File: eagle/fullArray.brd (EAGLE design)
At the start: 40 x 70 mm, 120 parts

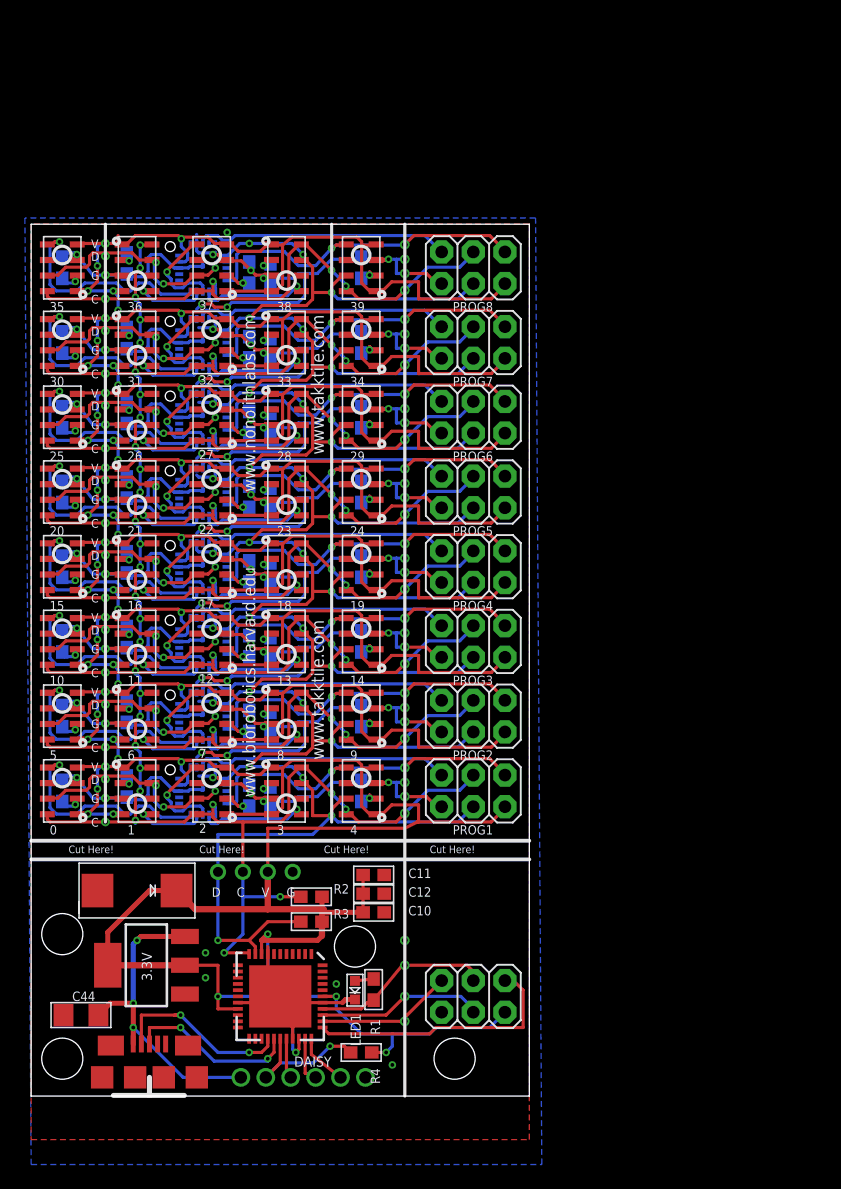
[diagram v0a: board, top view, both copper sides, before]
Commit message: need to tweak address pins, but should be manufacturable
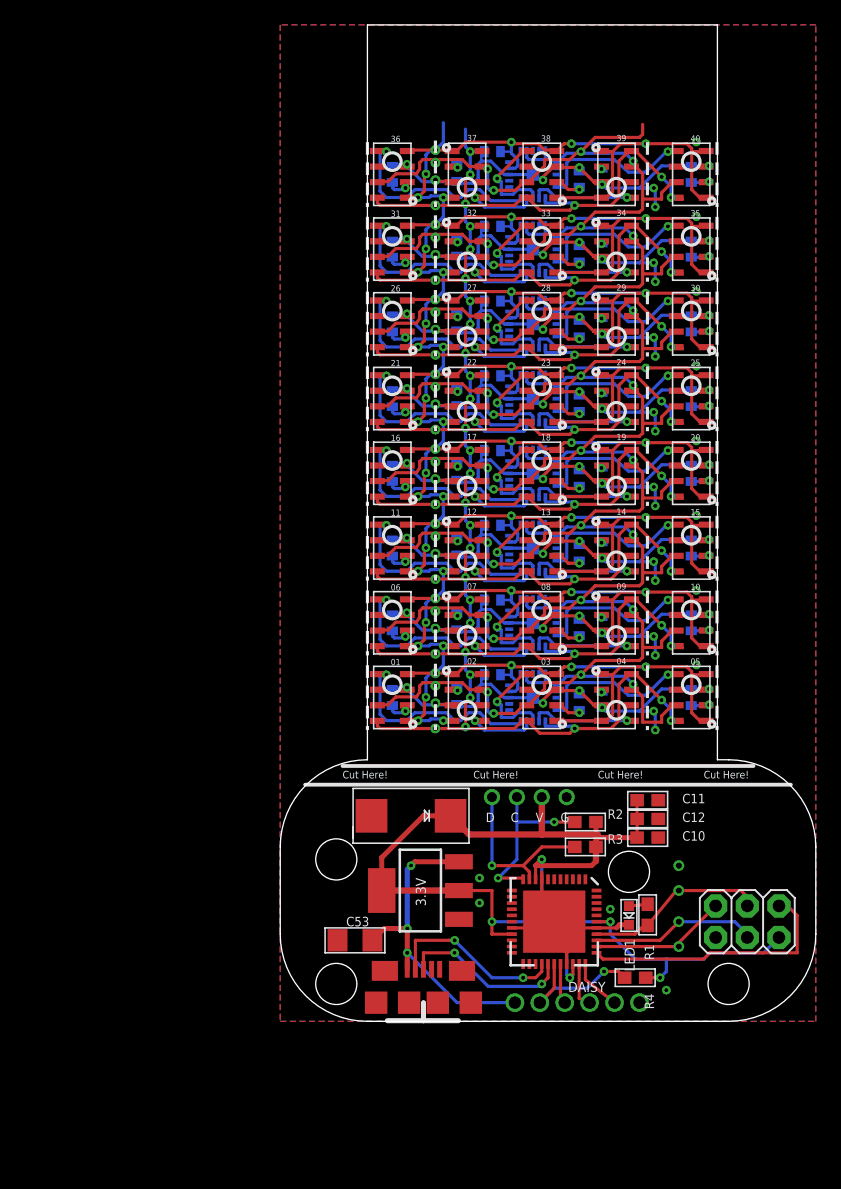
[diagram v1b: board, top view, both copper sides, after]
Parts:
- removed 0, 1, 2, 3, 4, 5, 6, 7, 8, 9: MPL115A2, nonolith:LGA-8
- removed AT1, AT2, AT3, AT4, AT5, AT6, AT7, AT8: ATTINYX4AMH, nonolith:QFN-20
- removed C0, C1, C2, C3, C4, C5, C7, C8, C9: 1uF, nonolith:0603
- removed PROG1, PROG2, PROG3, PROG4, PROG5, PROG6, PROG7, PROG8: (no value), nonolith:2X03
- added 01, 02, 03, 04, 05, 06, 07, 08, 09, 40: MPL115A, nonolith:LGA-8
- added C01, C02, C03, C04, C05, C07, C08, C09, C45, C46, C47, C48, C49, C50, C51: (no value), nonolith:0402
- added C52: 470uF, microbuilder:EIA7343-31/D-R
- added C53: 10uF, nonolith:1206
- added UC01, UC02, UC03, UC04, UC05, UC06, UC07, UC08: ATTINY24QFN, nonolith:QFN20
- 10, 11, 12, 13, 14, 15, 16, 17, 18, 19, 20, 21, 22, 23, 24, 25, 26, 27, 28, 29, 30, 31, 32, 33, 34, 35, 36, 37, 38, 39: value MPL115A2 -> MPL115A
- C13, C14, C15, C16, C17, C18, C19, C20, C21, C22, C23, C24, C25, C26, C27, C28, C29, C30, C31, C32, C33, C34, C35, C36, C37, C38, C39, C40, C41, C42, C6: value 1uF -> (none); device nonolith:0603 -> nonolith:0402
- C43: value 470uF -> (none); device microbuilder:EIA7343-31/D-R -> nonolith:0402
- C44: value 10uF -> (none); device nonolith:1206 -> nonolith:0402
- moved C44 78.6 mm to (33.0, 62.0), flipped to the bottom, turned to 90 degrees
- moved C43 63.5 mm to (25.8, 61.8), flipped to the bottom, turned to 270 degrees
- moved C38 50.7 mm to (33.0, 56.0)
- moved 10 50.5 mm to (33.0, 32.0)
- moved 15 50.5 mm to (33.0, 38.0)
- moved 20 50.5 mm to (33.0, 44.0)
- moved 25 50.5 mm to (33.0, 50.0)
- moved 30 50.5 mm to (33.0, 56.0)
- moved 35 50.5 mm to (33.0, 62.0)
- moved C14 45.3 mm to (33.0, 32.0), turned to 90 degrees
- moved C13 43.4 mm to (25.8, 31.8), turned to 270 degrees
- moved C18 41.5 mm to (24.0, 37.6)
- moved C19 38.2 mm to (25.8, 37.8)
- moved C24 36.3 mm to (24.0, 43.6), turned to 90 degrees
- moved C20 35.5 mm to (33.0, 38.0)
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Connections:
- removed net ADDR1: AT1.11
- removed net ADDR2: AT2.12
- removed net ADDR3: AT3.11, AT3.12
- removed net ADDR4: AT4.14
- removed net ADDR5: AT5.11, AT5.14
- removed net ADDR6: AT6.12, AT6.14
- removed net ADDR7: AT7.11, AT7.12, AT7.14
- removed net ADDR8: AT8.15
- removed net CAP00: 0.2, C0.1
- removed net RESET1: AT1.13, PROG1.5
- removed net RESET2: AT2.13, PROG2.5
- removed net RESET3: AT3.13, PROG3.5
- removed net RESET4: AT4.13, PROG4.5
- removed net RESET5: AT5.13, PROG5.5
- removed net RESET6: AT6.13, PROG6.5
- removed net RESET7: AT7.13, PROG7.5
- removed net RESET8: AT8.13, PROG8.5
- removed net RST18: 35.5, AT8.5
- removed net RST41: 3.5, AT1.2
- removed net RST42: 8.5, AT2.2
- removed net RST43: 13.5, AT3.2
- removed net RST44: 18.5, AT4.2
- removed net RST45: 23.5, AT5.2
- removed net RST46: 28.5, AT6.2
- removed net RST47: 33.5, AT7.2
- removed net RST48: 38.5, AT8.2
- removed net RST51: 4.5, AT1.20, PROG1.1
- removed net RST52: 9.5, AT2.20, PROG2.1
- removed net RST53: 14.5, AT3.20, PROG3.1
- removed net RST54: 19.5, AT4.20, PROG4.1
- removed net RST55: 24.5, AT5.20, PROG5.1
- removed net RST56: 29.5, AT6.20, PROG6.1
- removed net RST57: 34.5, AT7.20, PROG7.1
- removed net RST58: 39.5, AT8.20, PROG8.1
- new net ADDR00: UC01.11, UC02.11, UC03.11, UC04.11, UC05.11, UC06.11, UC07.11, UC08.11
- new net CAP39: 36.2, C46.1
- new net RESET01: UC01.13
- new net RESET02: UC02.13
- new net RESET03: UC03.13
- new net RESET04: UC04.13
- new net RESET05: UC05.13
- new net RESET06: UC06.13, UC07.13
- new net RESET08: UC08.13
- new net RST01: 01.5, UC01.5
- new net RST018: 18.5, UC04.3
- new net RST02: 02.5, UC01.4
- new net RST03: 03.5, UC01.3
- new net RST04: 04.5, UC01.2
- new net RST05: 05.5, UC01.20
- new net RST06: 06.5, UC02.5
- new net RST07: 07.5, UC02.4
- new net RST08: 08.5, UC02.3
- new net RST09: 09.5, UC02.2
- new net RST10: 10.5, UC02.20
- new net RST19: 19.5, UC04.2
- new net RST20: 20.5, UC04.20
- new net RST29: 29.5, UC06.2
- new net RST30: 30.5, UC06.20
- new net RST39: 39.5, UC08.2
- new net RST40: 40.5, UC08.20
- net 3.3V: now also 01.1, 01.4, 02.1, 02.4, 03.1, 03.4, 04.1, 04.4, 05.1, 05.4, 06.1, 06.4, 07.1, 07.4, 08.1, 08.4, 09.1, 09.4, 40.1, 40.4, C15.1, C21.1, C27.1, C33.1, C39.1, C45.1, C51.1, C52.+, C6.1, UC01.9, UC02.9, UC03.9, UC04.9, UC05.9, UC06.9, UC07.9, UC08.9; no longer 0.1, 0.4, 1.1, 1.4, 2.1, 2.4, 3.1, 3.4, 4.1, 4.4, 5.1, 5.4, 6.1, 6.4, 7.1, 7.4, 8.1, 8.4, 9.1, 9.4, AT1.9, AT2.9, AT3.9, AT4.9, AT5.9, AT6.9, AT7.9, AT8.9, C43.+, PROG1.2, PROG2.2, PROG3.2, PROG4.2, PROG5.2, PROG6.2, PROG7.2, PROG8.2
- net 5V: now also C53.2; no longer C44.2
- net CAP01: now also 01.2, C01.1; no longer 7.2, C7.1
- net CAP02: now also 02.2, C02.1; no longer 8.2, C8.1
- net CAP03: now also 03.2, C03.1; no longer 9.2, C9.1
- net CAP04: now also 04.2, C04.1; no longer 5.2, C5.1
- net CAP05: now also 05.2, C05.1; no longer 6.2, C6.1
- net CAP06: now also 08.2, C09.1; no longer 12.2, C15.1
- net CAP07: now also 09.2, C13.1; no longer 13.2, C16.1
- net CAP08: now also 10.2, C14.1; no longer 14.2, C17.1
- net CAP09: now also 06.2, C07.1; no longer 10.2, C13.1
- net CAP10: now also 07.2, C08.1; no longer 1.2, C1.1
- net CAP11: now also 13.2, C18.1; no longer 11.2, C14.1
- net CAP12: now also 14.2, C19.1; no longer 17.2, C20.1
- net CAP13: now also 15.2, C20.1; no longer 18.2, C21.1
- net CAP14: now also 11.2, C16.1; no longer 19.2, C22.1
- net CAP15: now also 12.2, C17.1; no longer 15.2, C18.1
- net CAP16: now also 18.2, C24.1; no longer 16.2, C19.1
- net CAP17: now also 19.2; no longer 22.2
- net CAP18: now also 20.2; no longer 23.2
- net CAP19: now also 16.2, C22.1; no longer 24.2, C27.1
- net CAP20: now also 17.2, C23.1; no longer 2.2, C2.1
- net CAP21: now also 23.2, C30.1; no longer 20.2, C23.1
- net CAP22: now also 24.2, C31.1; no longer 21.2, C24.1
- net CAP23: now also 25.2, C32.1; no longer 27.2, C30.1
- net CAP24: now also 21.2, C28.1; no longer 28.2, C31.1
- net CAP25: now also 22.2, C29.1; no longer 29.2, C32.1
- net CAP26: now also 28.2, C36.1; no longer 25.2, C28.1
- net CAP27: now also 29.2, C37.1; no longer 26.2, C29.1
- net CAP28: now also 30.2, C38.1; no longer 32.2, C35.1
- net CAP29: now also 26.2, C34.1; no longer 33.2, C36.1
- net CAP30: now also 27.2, C35.1; no longer 3.2, C3.1
- net CAP31: now also 33.2, C42.1; no longer 34.2, C37.1
- net CAP32: now also 34.2, C43.1; no longer 30.2, C33.1
- net CAP33: now also 35.2, C44.1; no longer 31.2, C34.1
- net CAP34: now also 31.2; no longer 37.2
- net CAP35: now also 32.2; no longer 38.2
- net CAP36: now also 38.2, C48.1; no longer 39.2, C42.1
- net CAP37: now also 39.2, C49.1; no longer 35.2, C38.1
- net CAP38: now also 40.2, C50.1; no longer 36.2, C39.1
- net CAP40: now also 37.2, C47.1; no longer 4.2, C4.1
- net GND: now also 01.3, 02.3, 03.3, 04.3, 05.3, 06.3, 07.3, 08.3, 09.3, 40.3, C01.2, C02.2, C03.2, C04.2, C05.2, C07.2, C08.2, C09.2, C43.2, C44.2, C45.2, C46.2, C47.2, C48.2, C49.2, C50.2, C51.2, C52.-, C53.1, UC01.0, UC01.12, UC01.14, UC01.15, UC01.8, UC02.0, UC02.12, UC02.14, UC02.15, UC02.8, UC03.0, UC03.12, UC03.14, UC03.15, UC03.8, UC04.0, UC04.12, UC04.14, UC04.15, UC04.8, UC05.0, UC05.12, UC05.14, UC05.15, UC05.8, UC06.0, UC06.12, UC06.14, UC06.15, UC06.8, UC07.0, UC07.12, UC07.14, UC07.15, UC07.8, UC08.0, UC08.12, UC08.14, UC08.15, UC08.8; no longer 0.3, 1.3, 2.3, 3.3, 4.3, 5.3, 6.3, 7.3, 8.3, 9.3, AT1.12, AT1.14, AT1.15, AT1.8, AT2.11, AT2.14, AT2.15, AT2.8, AT3.14, AT3.15, AT3.8, AT4.11, AT4.12, AT4.15, AT4.8, AT5.12, AT5.15, AT5.8, AT6.11, AT6.15, AT6.8, AT7.15, AT7.8, AT8.11, AT8.12, AT8.14, AT8.8, C0.2, C1.2, C2.2, C3.2, C4.2, C43.-, C44.1, C5.2, C7.2, C8.2, C9.2, PROG1.6, PROG2.6, PROG3.6, PROG4.6, PROG5.6, PROG6.6, PROG7.6, PROG8.6
- net RST11: now also 11.5, UC03.5; no longer 0.5, AT1.5
- net RST12: now also 12.5, UC03.4; no longer 5.5, AT2.5
- net RST13: now also 13.5, UC03.3; no longer 10.5, AT3.5
- net RST14: now also 14.5, UC03.2; no longer 15.5, AT4.5
- net RST15: now also 15.5, UC03.20; no longer 20.5, AT5.5
- net RST16: now also 16.5, UC04.5; no longer 25.5, AT6.5
- net RST17: now also 17.5, UC04.4; no longer 30.5, AT7.5
- net RST21: now also 21.5, UC05.5; no longer 1.5, AT1.4
- net RST22: now also 22.5, UC05.4; no longer 6.5, AT2.4
- net RST23: now also 23.5, UC05.3; no longer 11.5, AT3.4
- net RST24: now also 24.5, UC05.2; no longer 16.5, AT4.4
- net RST25: now also 25.5, UC05.20; no longer 21.5, AT5.4
- net RST26: now also UC06.5; no longer AT6.4
- net RST27: now also 27.5, UC06.4; no longer 31.5, AT7.4
- net RST28: now also 28.5, UC06.3; no longer 36.5, AT8.4
- net RST31: now also 31.5, UC07.5; no longer 2.5, AT1.3
- net RST32: now also 32.5, UC07.4; no longer 7.5, AT2.3
- net RST33: now also 33.5, UC07.3; no longer 12.5, AT3.3
- net RST34: now also 34.5, UC07.2; no longer 17.5, AT4.3
- net RST35: now also 35.5, UC07.20; no longer 22.5, AT5.3
- net RST36: now also 36.5, UC08.5; no longer 27.5, AT6.3
- net RST37: now also 37.5, UC08.4; no longer 32.5, AT7.3
- net RST38: now also 38.5, UC08.3; no longer 37.5, AT8.3
- net SCL: now also 01.8, 02.8, 03.8, 04.8, 05.8, 06.8, 07.8, 08.8, 09.8, 40.8, UC01.1, UC02.1, UC03.1, UC04.1, UC05.1, UC06.1, UC07.1, UC08.1; no longer 0.8, 1.8, 2.8, 3.8, 4.8, 5.8, 6.8, 7.8, 8.8, 9.8, AT1.1, AT2.1, AT3.1, AT4.1, AT5.1, AT6.1, AT7.1, AT8.1, PROG1.3, PROG2.3, PROG3.3, PROG4.3, PROG5.3, PROG6.3, PROG7.3, PROG8.3
- net SDA: now also 01.7, 02.7, 03.7, 04.7, 05.7, 06.7, 07.7, 08.7, 09.7, 40.7, UC01.16, UC02.16, UC03.16, UC04.16, UC05.16, UC06.16, UC07.16, UC08.16; no longer 0.7, 1.7, 2.7, 3.7, 4.7, 5.7, 6.7, 7.7, 8.7, 9.7, AT1.16, AT2.16, AT3.16, AT4.16, AT5.16, AT6.16, AT7.16, AT8.16, PROG1.4, PROG2.4, PROG3.4, PROG4.4, PROG5.4, PROG6.4, PROG7.4, PROG8.4
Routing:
- net GND: track 493.3 -> 368.6 mm, vias 84 -> 77
- net SDA: track 439.6 -> 353.9 mm, vias 57 -> 41
- net SCL: track 445.9 -> 365.8 mm, vias 66 -> 58
- net 3.3V: track 636.8 -> 574.4 mm, vias 52 -> 61
- net RST55: track 27.8 -> 0.00 mm, vias 2 -> 0
- net RST54: track 27.8 -> 0.00 mm, vias 2 -> 0
- net RST58: track 27.8 -> 0.00 mm, vias 2 -> 0
- net RST57: track 27.8 -> 0.00 mm, vias 2 -> 0
- net RST56: track 27.8 -> 0.00 mm, vias 2 -> 0
- net RST53: track 27.8 -> 0.00 mm, vias 2 -> 0
- net RST52: track 27.8 -> 0.00 mm, vias 2 -> 0
- net RST51: track 27.8 -> 0.00 mm, vias 2 -> 0
- net RESET4: track 20.6 -> 0.00 mm
- net RESET2: track 20.6 -> 0.00 mm
- net RESET8: track 20.6 -> 0.00 mm
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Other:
- board size 40 x 70 mm -> 43 x 80 mm
- board text removed: "www.biorobotics.harvard.edu"
- board text removed: "www.nonolithlabs.com"
- board text removed: "www.takktile.com"
